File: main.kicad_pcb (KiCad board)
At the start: 2 copper layers, 23 parts, among them J1 Conn_01x02_Socket, U1 ESP32-WROOM-32, U2 LM324

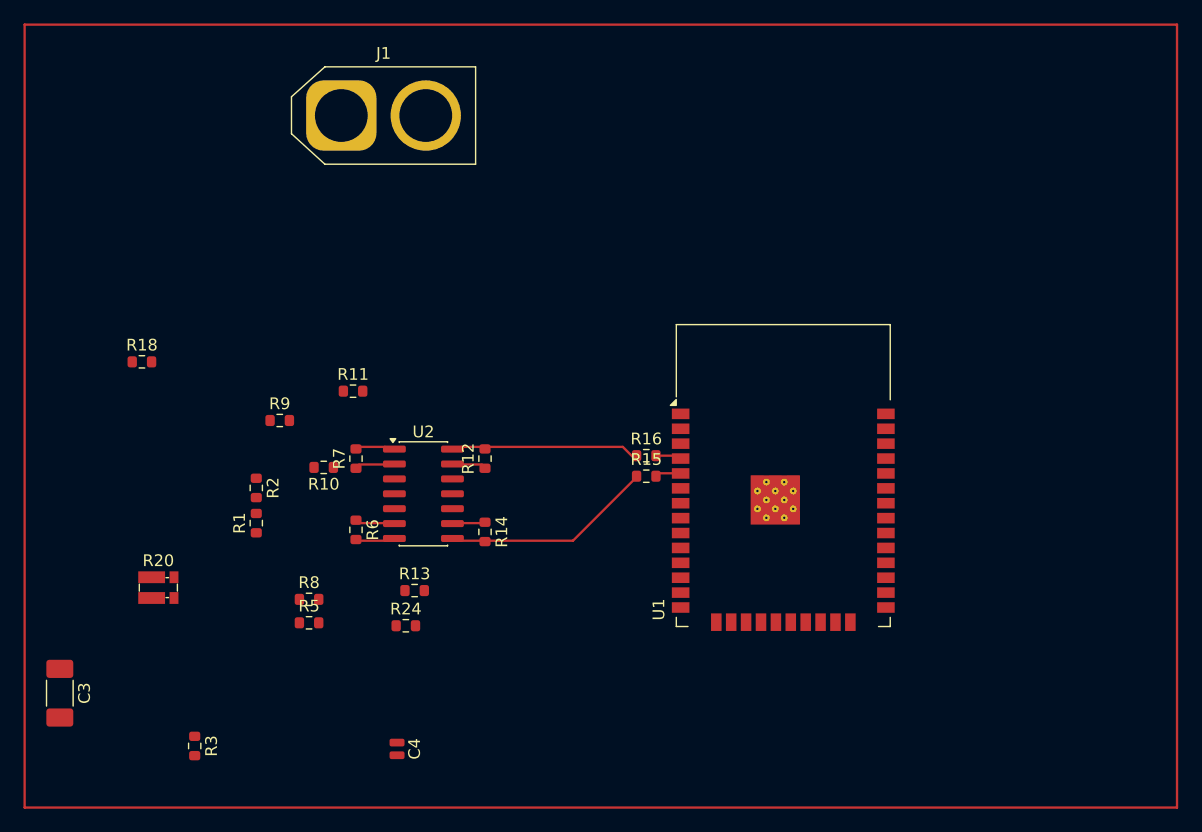
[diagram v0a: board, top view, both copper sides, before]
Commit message: make PCB layout
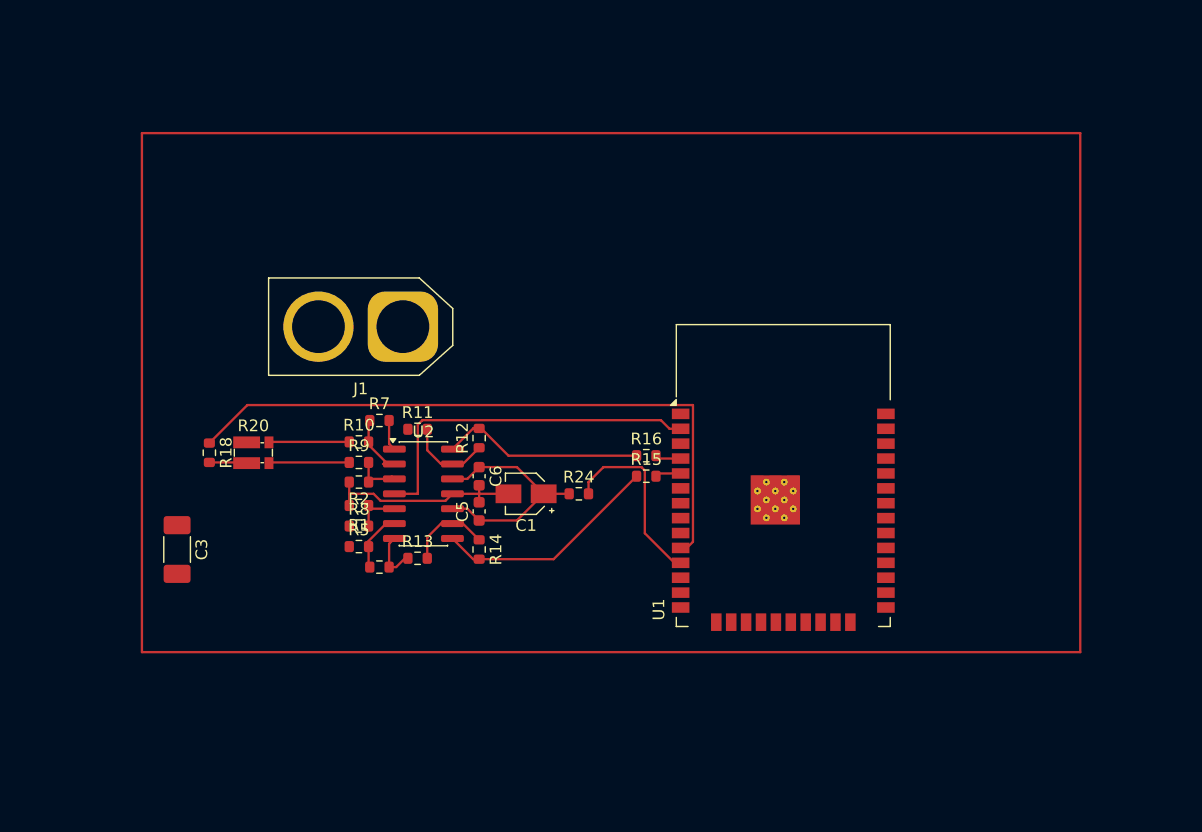
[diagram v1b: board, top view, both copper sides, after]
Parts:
- removed C4: C_Small, Capacitor_SMD:C_0504_1310Metric
- removed R3: 10R, Resistor_SMD:R_0603_1608Metric
- added C1: C_Polarized, Capacitor_SMD:CP_Elec_3x5.3, F.Cu at (145.2, 86.5)
- added C5: C_Small, Capacitor_SMD:C_0603_1608Metric, F.Cu at (141.2, 88.0)
- added C6: C_Small, Capacitor_SMD:C_0603_1608Metric, F.Cu at (141.2, 85.0)
- moved J1 18.8 mm to (134.8, 72.2), turned to 180 degrees
- moved R24 18.6 mm to (149.8, 86.5)
- moved C3 15.8 mm to (115.5, 91.2)
- moved R20 14.1 mm to (122.0, 83.0)
- moved R18 9.65 mm to (118.2, 83.0), turned to -90 degrees
- moved R1 8.88 mm to (131.0, 87.5), turned to 180 degrees
- moved R2 8.76 mm to (131.0, 85.5), turned to 180 degrees
- moved R5 7.77 mm to (131.0, 91.0)
- moved R9 7.64 mm to (131.0, 83.8)
- moved R8 7.56 mm to (131.0, 89.2)
- moved R11 6.39 mm to (136.0, 81.0)
- moved R7 3.82 mm to (132.8, 80.2), turned to 0 degrees
- moved R6 3.75 mm to (132.8, 92.8), turned to 0 degrees
- moved R10 3.71 mm to (131.0, 82.1), turned to 0 degrees
- moved R13 2.76 mm to (136.0, 92.0)
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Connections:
- C3 pad 2: Net-(C3-Pad2) -> GND
- R1 pad 2: Net-(C4-Pad1) -> GND
- R10 pad 1: Net-(C3-Pad2) -> Net-(R10-Pad1)
- R11 pad 1: Net-(C4-Pad1) -> Net-(R11-Pad1)
- R13 pad 1: Net-(C4-Pad1) -> Net-(R13-Pad1)
- R2 pad 2: Net-(C4-Pad1) -> GND
- R20 pad 1: Net-(R18-Pad2) -> Net-(C3-Pad1)
- R20 pad 2: Net-(R20-Pad2) -> Net-(R10-Pad1)
- R20 pad 4: Net-(C3-Pad1) -> Net-(R18-Pad2)
- R24 pad 1: Net-(C4-Pad1) -> Net-(U2C-+)
- R5 pad 1: Net-(R20-Pad3) -> GND
- R6 pad 2: Net-(U2C-+) -> Net-(R13-Pad1)
- R7 pad 2: Net-(U2D-+) -> Net-(R11-Pad1)
- R8 pad 1: Net-(R20-Pad2) -> Net-(C3-Pad1)
- R9 pad 1: Net-(C3-Pad1) -> Net-(R20-Pad3)
- U2 pad 1: Net-(U2D-+) -> Net-(R11-Pad1)
- U2 pad 12: Net-(U2D-+) -> Net-(U2C-+)
- U2 pad 7: Net-(U2C-+) -> Net-(R13-Pad1)
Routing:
- net /DAC_Sinus: track 0.00 -> 55.5 mm
- net VDD: track 0.00 -> 30.8 mm
- net Net-(U2C-+): track 0.00 -> 20.4 mm
- net Net-(R14-Pad2): track 0.00 -> 19.4 mm
- net GND: track 0.00 -> 17.5 mm
- net Net-(R12-Pad2): track 0.00 -> 17.4 mm
- net /DAC_Amp_offcet: track 0.00 -> 15.9 mm
- net Net-(U2C--): track 0.00 -> 7.92 mm
- net Net-(U2D--): track 0.00 -> 7.27 mm
- net Net-(R20-Pad3): track 0.00 -> 6.87 mm
- net Net-(R10-Pad1): track 0.00 -> 6.86 mm
- net Net-(U2A--): track 0.00 -> 5.97 mm
- net Net-(U2B--): track 0.00 -> 5.19 mm
- net Net-(R13-Pad1): track 0.00 -> 4.54 mm
- net Net-(U2A-+): track 0.00 -> 4.31 mm
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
